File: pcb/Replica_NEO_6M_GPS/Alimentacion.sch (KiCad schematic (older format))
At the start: 7 parts, among them U1 TPS79133DBVR

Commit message: Se acomodaron archivos y se hicieron retoques
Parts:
- U1: symbol TPS79133DBVR:TPS79133DBVR -> Replica_NEO_6M_GPS-rescue:TPS79133DBVR-TPS79133DBVR
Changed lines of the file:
@@
 $EndDescr
 $Comp
-L TPS79133DBVR:TPS79133DBVR U1
+L Replica_NEO_6M_GPS-rescue:TPS79133DBVR-TPS79133DBVR U1
 U 1 1 60ECBB96
 P 5550 3450

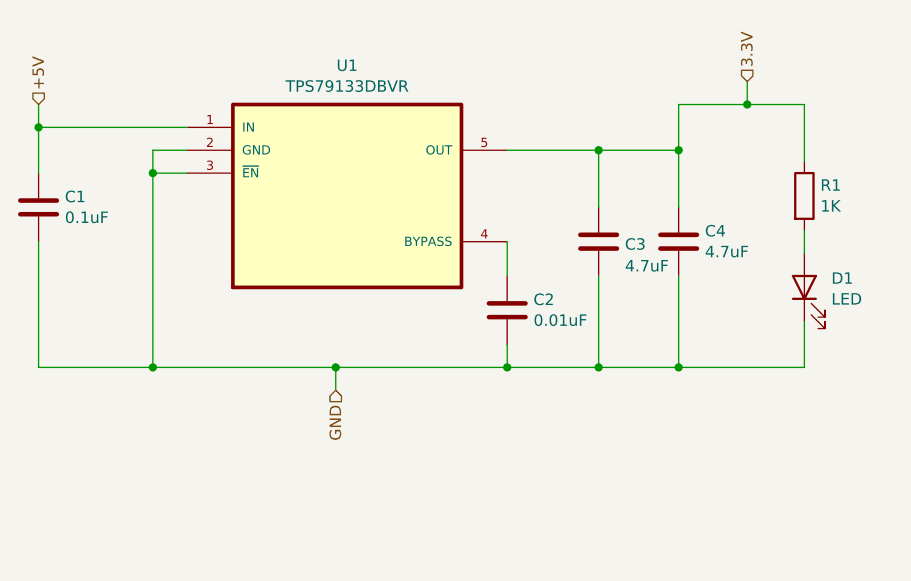
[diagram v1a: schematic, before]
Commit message: se retoco el esquematico
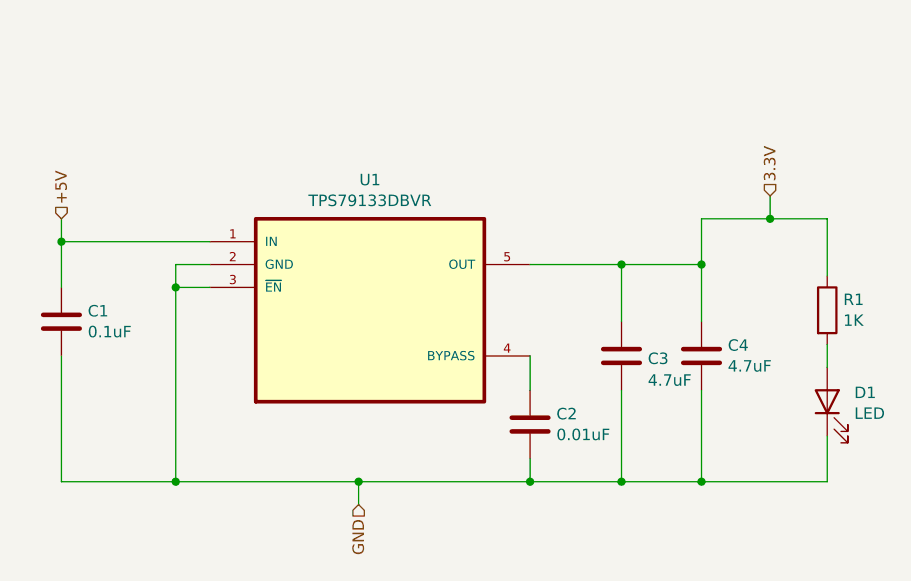
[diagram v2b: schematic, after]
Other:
- moved on the sheet: C1, C2, C3, C4, D1, R1, U1
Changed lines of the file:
@@
 L Replica_NEO_6M_GPS-rescue:TPS79133DBVR-TPS79133DBVR U1
 U 1 1 60ECBB96
-P 5550 3450
-F 0 "U1" H 5550 4020 50  0000 C CNN
-F 1 "TPS79133DBVR" H 5550 3929 50  0000 C CNN
-F 2 "TPS79133DBVR:SOT95P280X145-5N" H 5550 3450 50  0001 L BNN
-F 3 "" H 5550 3450 50  0001 L BNN
-	1    5550 3450
+P 5650 3950
+F 0 "U1" H 5650 4520 50  0000 C CNN
+F 1 "TPS79133DBVR" H 5650 4429 50  0000 C CNN
+F 2 "TPS79133DBVR:SOT95P280X145-5N" H 5650 3950 50  0001 L BNN
+F 3 "" H 5650 3950 50  0001 L BNN
+	1    5650 3950
 	1    0    0    -1
 $EndComp
@@
 L Device:C C1
 U 1 1 60ECC43D
-P 4200 3500
-F 0 "C1" H 4315 3546 50  0000 L CNN
-F 1 "0.1uF" H 4315 3455 50  0000 L CNN
-F 2 "Capacitor_SMD:C_0805_2012Metric_Pad1.18x1.45mm_HandSolder" H 4238 3350 50  0001 C CNN
-F 3 "~" H 4200 3500 50  0001 C CNN
-	1    4200 3500
+P 4300 4000
+F 0 "C1" H 4415 4046 50  0000 L CNN
+F 1 "0.1uF" H 4415 3955 50  0000 L CNN
+F 2 "Capacitor_SMD:C_0805_2012Metric_Pad1.18x1.45mm_HandSolder" H 4338 3850 50  0001 C CNN
+F 3 "~" H 4300 4000 50  0001 C CNN
+	1    4300 4000
 	1    0    0    -1
 $EndComp
@@
 L Device:C C2
 U 1 1 60ECCA14
-P 6250 3950
-F 0 "C2" H 6365 3996 50  0000 L CNN
-F 1 "0.01uF" H 6365 3905 50  0000 L CNN
-F 2 "Capacitor_SMD:C_0805_2012Metric_Pad1.18x1.45mm_HandSolder" H 6288 3800 50  0001 C CNN
-F 3 "~" H 6250 3950 50  0001 C CNN
-	1    6250 3950
+P 6350 4450
+F 0 "C2" H 6465 4496 50  0000 L CNN
+F 1 "0.01uF" H 6465 4405 50  0000 L CNN
+F 2 "Capacitor_SMD:C_0805_2012Metric_Pad1.18x1.45mm_HandSolder" H 6388 4300 50  0001 C CNN
+F 3 "~" H 6350 4450 50  0001 C CNN
+	1    6350 4450
 	1    0    0    -1
 $EndComp
@@
 L Device:C C3
 U 1 1 60ECD2B3
-P 6650 3650
-F 0 "C3" H 6765 3638 50  0000 L CNN
-F 1 "4.7uF" H 6765 3543 50  0000 L CNN
-F 2 "Capacitor_SMD:C_0805_2012Metric_Pad1.18x1.45mm_HandSolder" H 6688 3500 50  0001 C CNN
-F 3 "~" H 6650 3650 50  0001 C CNN
-	1    6650 3650
+P 6750 4150
+F 0 "C3" H 6865 4138 50  0000 L CNN
+F 1 "4.7uF" H 6865 4043 50  0000 L CNN
+F 2 "Capacitor_SMD:C_0805_2012Metric_Pad1.18x1.45mm_HandSolder" H 6788 4000 50  0001 C CNN
+F 3 "~" H 6750 4150 50  0001 C CNN
+	1    6750 4150
 	1    0    0    -1
 $EndComp
@@
 L Device:C C4
 U 1 1 60ECD89A
-P 7000 3650
-F 0 "C4" H 7115 3696 50  0000 L CNN
-F 1 "4.7uF" H 7115 3605 50  0000 L CNN
-F 2 "Capacitor_SMD:C_0805_2012Metric_Pad1.18x1.45mm_HandSolder" H 7038 3500 50  0001 C CNN
-F 3 "~" H 7000 3650 50  0001 C CNN
-	1    7000 3650
+P 7100 4150
+F 0 "C4" H 7215 4196 50  0000 L CNN
+F 1 "4.7uF" H 7215 4105 50  0000 L CNN
+F 2 "Capacitor_SMD:C_0805_2012Metric_Pad1.18x1.45mm_HandSolder" H 7138 4000 50  0001 C CNN
+F 3 "~" H 7100 4150 50  0001 C CNN
+	1    7100 4150
 	1    0    0    -1
 $EndComp
@@
 L Device:R R1
 U 1 1 60ED22D6
-P 7550 3450
-F 0 "R1" H 7620 3496 50  0000 L CNN
-F 1 "1K" H 7620 3405 50  0000 L CNN
-F 2 "Resistor_SMD:R_0805_2012Metric_Pad1.20x1.40mm_HandSolder" V 7480 3450 50  0001 C CNN
-F 3 "~" H 7550 3450 50  0001 C CNN
-	1    7550 3450
+P 7650 3950
+F 0 "R1" H 7720 3996 50  0000 L CNN
+F 1 "1K" H 7720 3905 50  0000 L CNN
+F 2 "Resistor_SMD:R_0805_2012Metric_Pad1.20x1.40mm_HandSolder" V 7580 3950 50  0001 C CNN
+F 3 "~" H 7650 3950 50  0001 C CNN
+	1    7650 3950
 	1    0    0    -1
 $EndComp
@@
 L Device:LED D1
 U 1 1 60ED357F
-P 7550 3850
-F 0 "D1" V 7589 3732 50  0000 R CNN
-F 1 "LED" V 7498 3732 50  0000 R CNN
-F 2 "LED_SMD:LED_0805_2012Metric_Pad1.15x1.40mm_HandSolder" H 7550 3850 50  0001 C CNN
-F 3 "~" H 7550 3850 50  0001 C CNN
-	1    7550 3850
+P 7650 4350
+F 0 "D1" V 7689 4232 50  0000 R CNN
+F 1 "LED" V 7598 4232 50  0000 R CNN
+F 2 "LED_SMD:LED_0805_2012Metric_Pad1.15x1.40mm_HandSolder" H 7650 4350 50  0001 C CNN
+F 3 "~" H 7650 4350 50  0001 C CNN
+	1    7650 4350
 	0    -1   -1   0
 $EndComp
 Wire Wire Line
-	6250 3250 6650 3250
+	6350 3750 6750 3750
 Wire Wire Line
-	7000 3250 7000 3500
+	7100 3750 7100 4000
 Wire Wire Line
-	6650 3250 6650 3500
-Connection ~ 6650 3250
+	6750 3750 6750 4000
+Connection ~ 6750 3750
 Wire Wire Line
-	6650 3250 7000 3250
+	6750 3750 7100 3750
 Wire Wire Line
-	6250 3650 6250 3800
+	6350 4150 6350 4300
 Wire Wire Line
-	6250 4100 6250 4200
+	6350 4600 6350 4700
 Wire Wire Line
-	6650 3800 6650 4200
+	6750 4300 6750 4700
 Wire Wire Line
-	7000 3800 7000 4200
+	7100 4300 7100 4700
 Wire Wire Line
-	7550 3600 7550 3700
+	7650 4100 7650 4200
 Wire Wire Line
-	7550 4000 7550 4200
+	7650 4500 7650 4700
 Wire Wire Line
-	4850 3250 4700 3250
+	4950 3750 4800 3750
 Wire Wire Line
-	4700 3250 4700 3350
+	4800 3750 4800 3850
 Wire Wire Line
-	4850 3350 4700 3350
-Connection ~ 4700 3350
+	4950 3850 4800 3850
+Connection ~ 4800 3850
 Wire Wire Line
-	4700 3350 4700 4200
+	4800 3850 4800 4700
 Wire Wire Line
-	4200 3150 4200 3350
+	4300 3650 4300 3850
 Wire Wire Line
-	4200 3650 4200 4200
+	4300 4150 4300 4700
 Wire Wire Line
-	7550 3050 7550 3300
+	7650 3550 7650 3800
 Wire Wire Line
-	7000 3050 7000 3250
-Connection ~ 7000 3250
+	7100 3550 7100 3750
+Connection ~ 7100 3750
 Wire Wire Line
-	4200 3050 4200 3150
-Connection ~ 4200 3150
-Text HLabel 7300 2950 1    50   Input ~ 0
+	4300 3550 4300 3650
+Connection ~ 4300 3650
+Text HLabel 7400 3450 1    50   Input ~ 0
 3.3V
 Wire Wire Line
-	7000 3050 7300 3050
+	7100 3550 7400 3550
 Wire Wire Line
-	7300 3050 7300 2950
-Connection ~ 7300 3050
+	7400 3550 7400 3450
+Connection ~ 7400 3550
 Wire Wire Line
-	7300 3050 7550 3050
-Text HLabel 4200 3050 1    50   Input ~ 0
+	7400 3550 7650 3550
+Text HLabel 4300 3550 1    50   Input ~ 0
 +5V
-Text HLabel 5500 4300 3    50   Input ~ 0
+Text HLabel 5600 4800 3    50   Input ~ 0
 GND
 Wire Wire Line
-	4200 4200 4700 4200
+	4300 4700 4800 4700
 Wire Wire Line
-	4700 4200 5500 4200
-Connection ~ 4700 4200
+	4800 4700 5600 4700
+Connection ~ 4800 4700
 Wire Wire Line
-	6250 4200 6650 4200
-Connection ~ 6250 4200
+	6350 4700 6750 4700
+Connection ~ 6350 4700
 Wire Wire Line
-	6650 4200 7000 4200
-Connection ~ 6650 4200
+	6750 4700 7100 4700
+Connection ~ 6750 4700
 Wire Wire Line
-	7000 4200 7550 4200
-Connection ~ 7000 4200
+	7100 4700 7650 4700
+Connection ~ 7100 4700
 Wire Wire Line
-	5500 4300 5500 4200
-Connection ~ 5500 4200
+	5600 4800 5600 4700
+Connection ~ 5600 4700
 Wire Wire Line
-	5500 4200 6250 4200
+	5600 4700 6350 4700
 Wire Wire Line
-	4200 3150 4850 3150
+	4300 3650 4950 3650
 $EndSCHEMATC
